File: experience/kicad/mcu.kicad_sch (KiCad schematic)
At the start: 38 parts, among them J1 USB_C_Receptacle_USB2.0_16P, U1 RP2040, U3 TPS54302

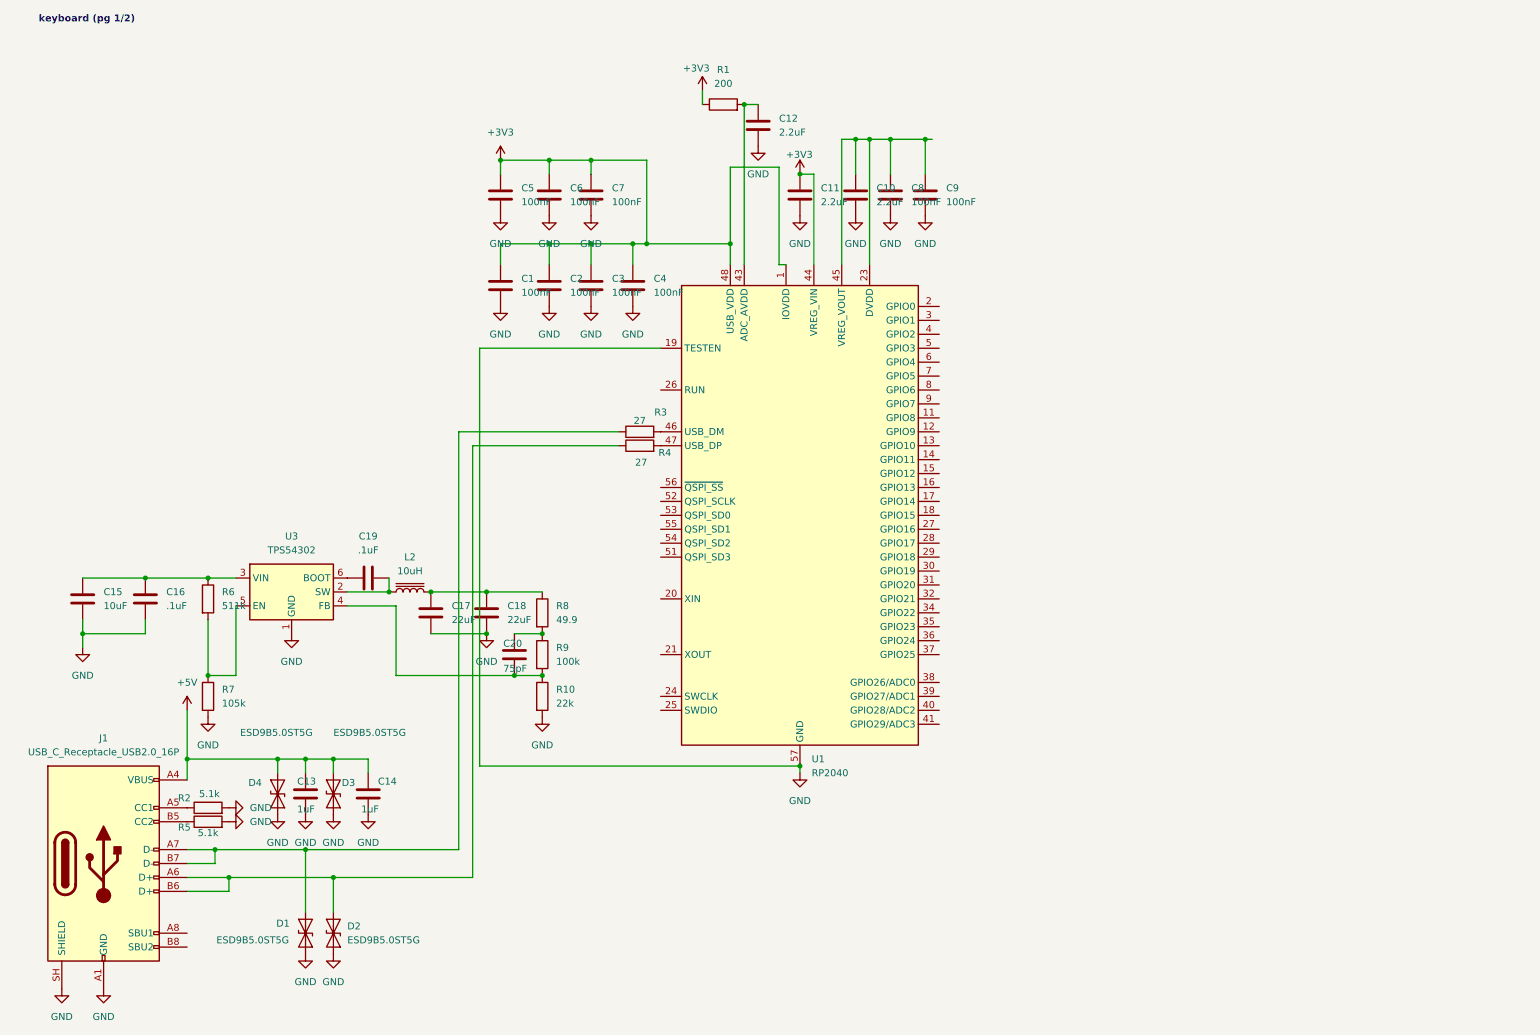
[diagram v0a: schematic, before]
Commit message: keyboard
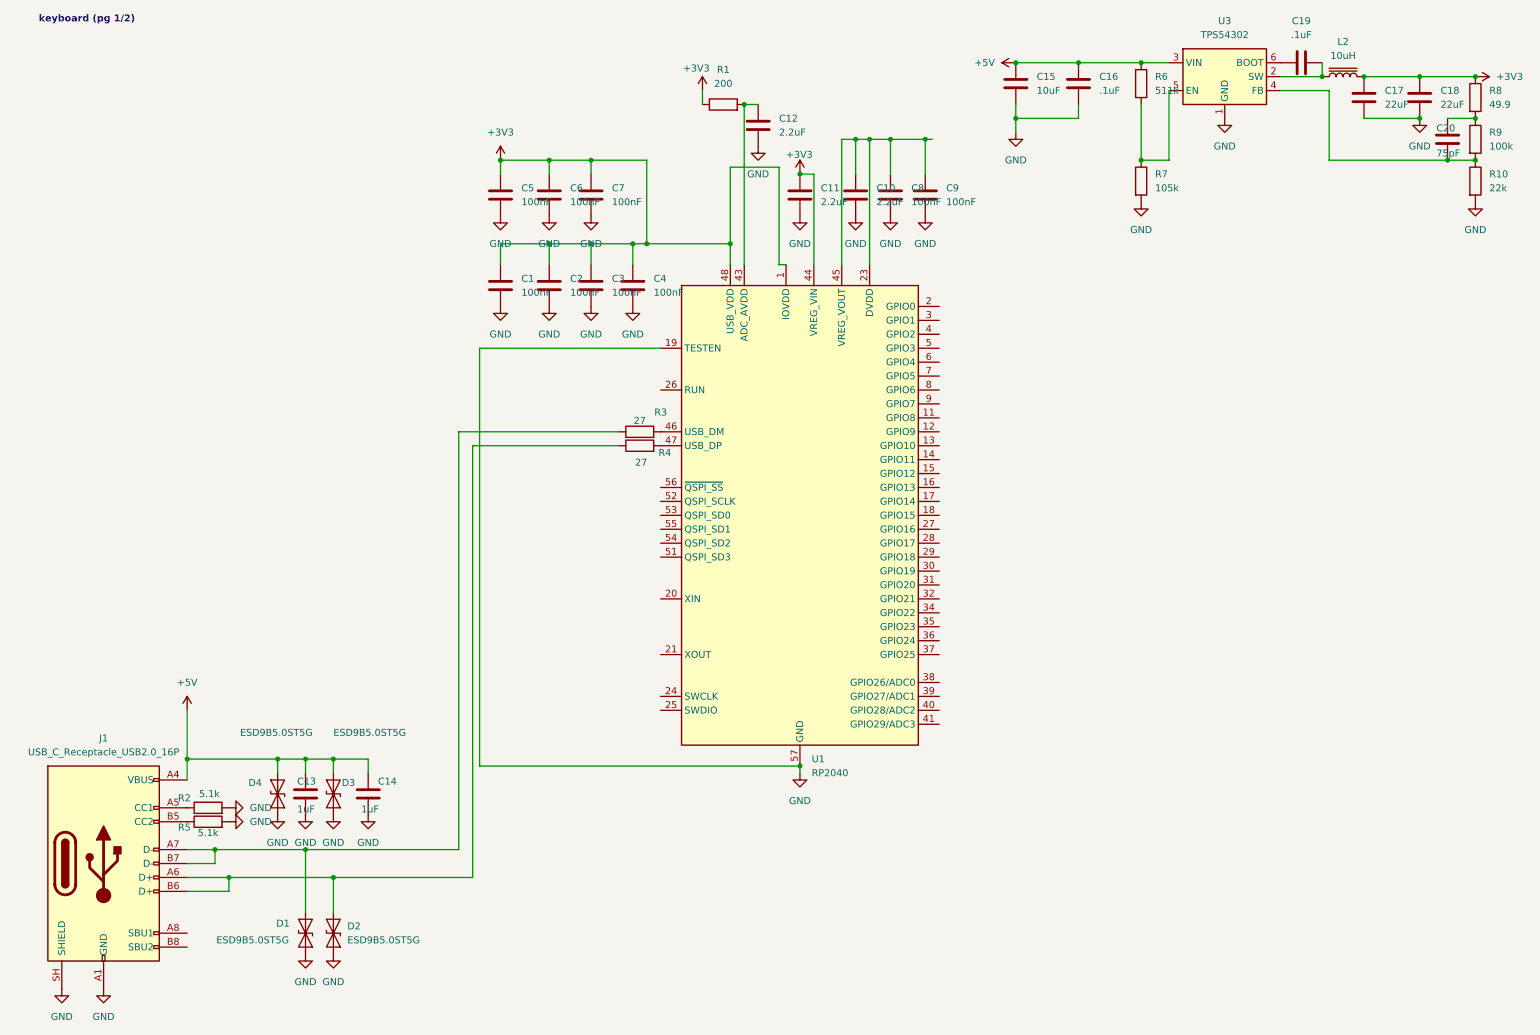
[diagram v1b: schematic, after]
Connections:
- net +3V3: now also C17.1, C18.1, L2.2, R8.1
- net +5V: now also C15.1, C16.1, R6.1, U3.3 (VIN)
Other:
- moved on the sheet: C15, C16, C17, C18, C19, C20, L2, R10, R6, R7, R8, R9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
